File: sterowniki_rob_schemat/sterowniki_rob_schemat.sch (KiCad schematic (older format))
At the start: 6 parts, among them Q1 Q_NPN_BCE, U1 STM32L476VGTx

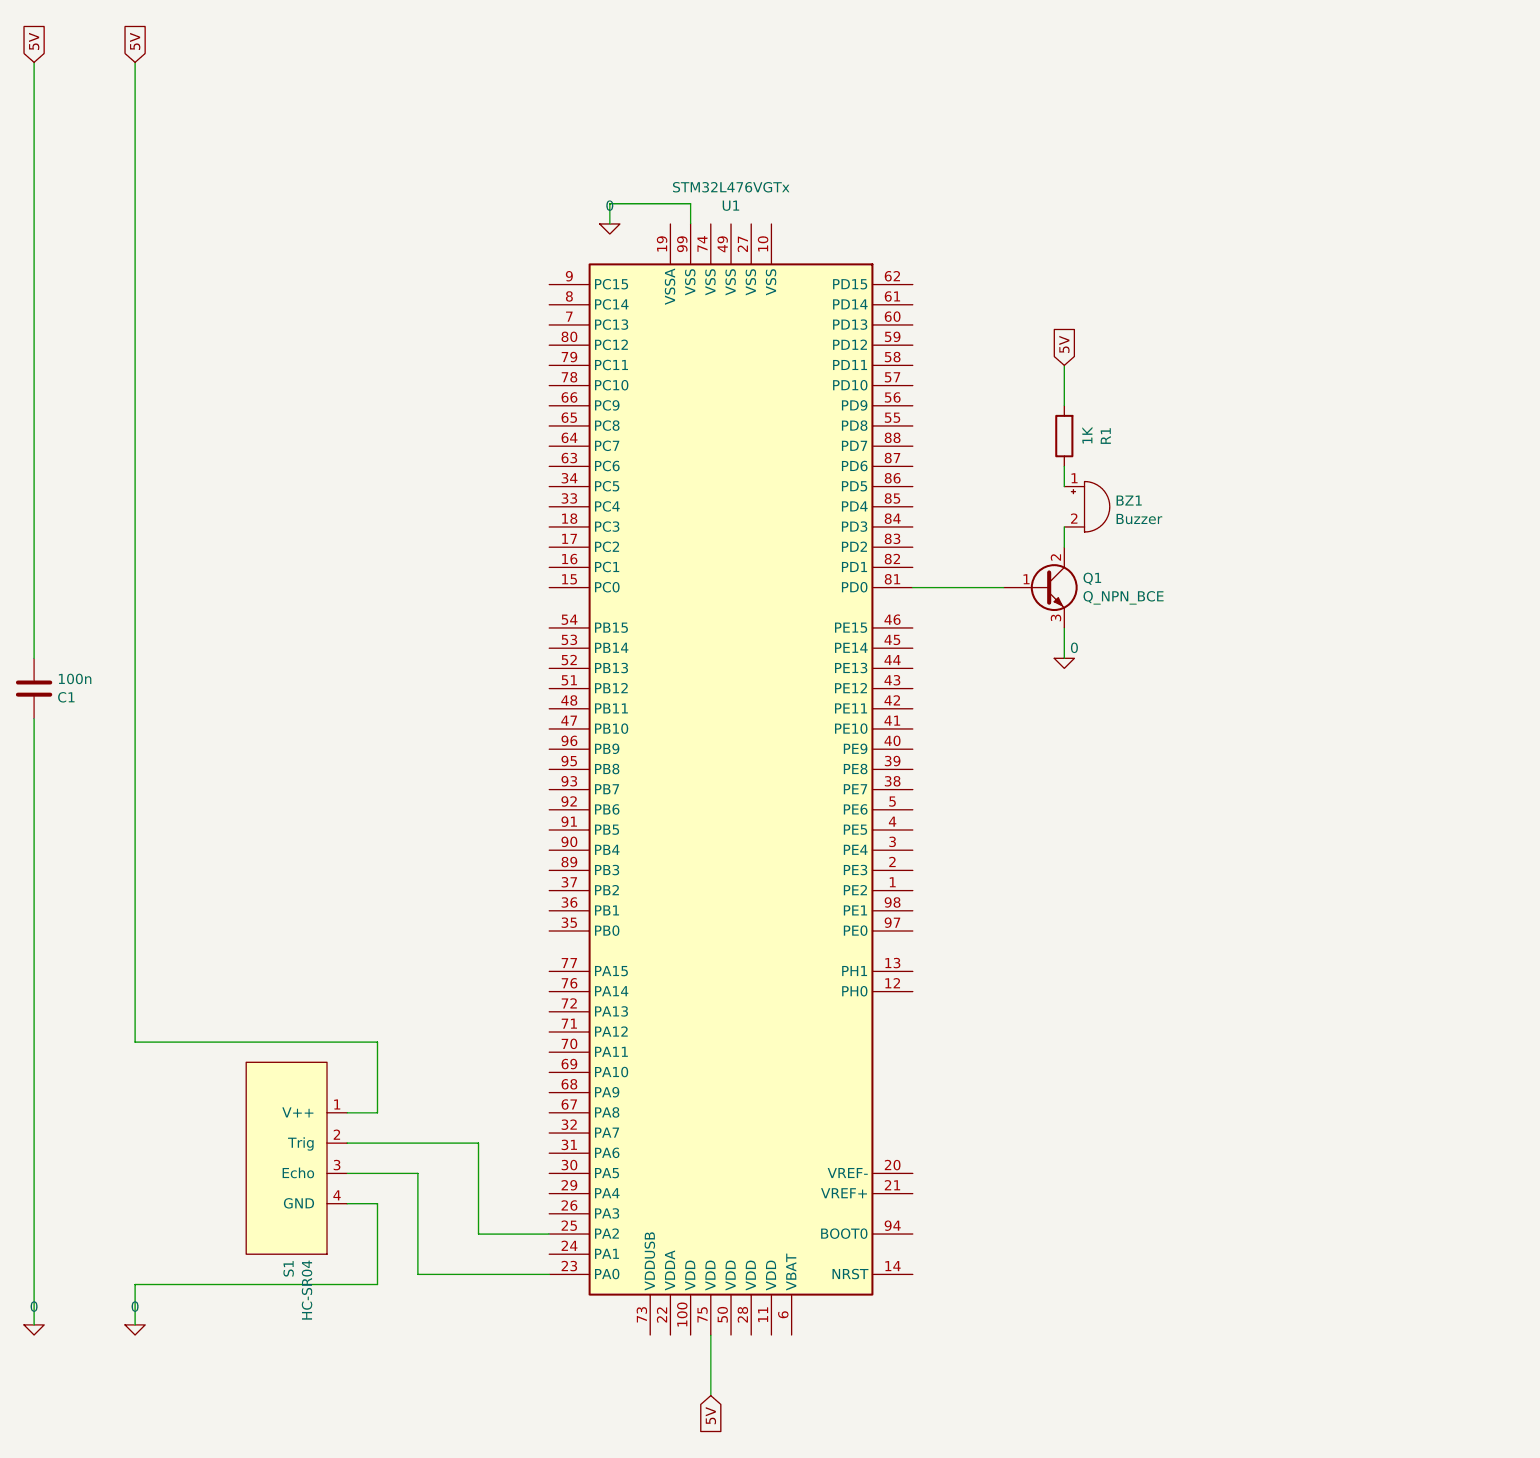
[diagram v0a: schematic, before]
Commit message: końcowy schemat układu
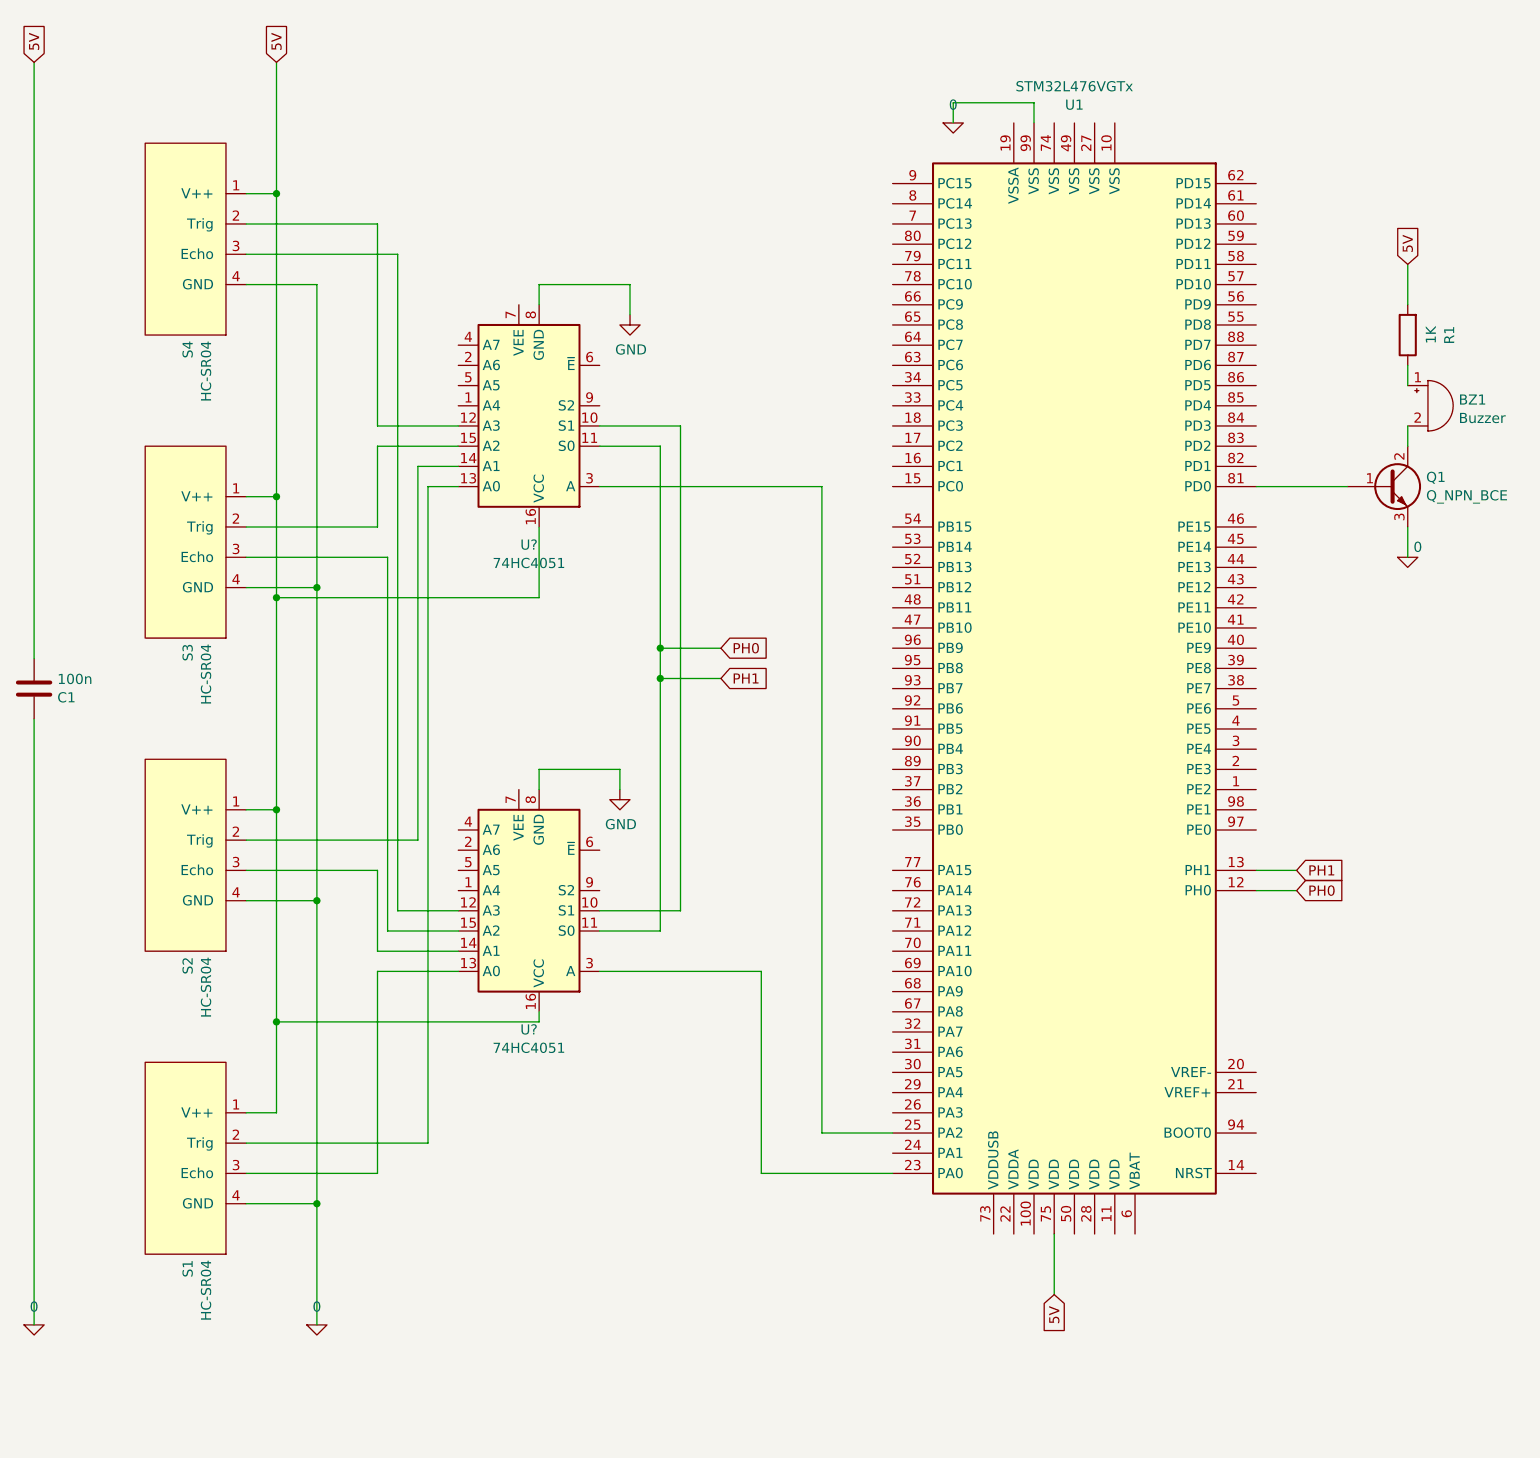
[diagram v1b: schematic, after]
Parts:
- added S2, S3, S4: HC-SR04, symbol bib:HC-SR04
- added U? (x2): 74HC4051, symbol 74xx:74HC4051
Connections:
- net 0: now also S2.4 (GND), S3.4 (GND), S4.4 (GND)
- net 5V: now also S2.1 (V++), S3.1 (V++), S4.1 (V++), U?.16 (VCC), U?.16 (VCC)
- net at S1.2 (Trig): now also U?.13 (A0); no longer U1.25 (PA2)
- net at S1.3 (Echo): now also U?.13 (A0); no longer U1.23 (PA0)
- net PH0: now reaches U1.12 (PH0)
- net PH0: now also U1.13 (PH1), U?.11 (S0), U?.11 (S0)
- new net: U1.23 (PA0), U?.3 (A)
- new net: U1.25 (PA2), U?.3 (A)
- new net: S2.2 (Trig), U?.14 (A1)
- new net: S2.3 (Echo), U?.14 (A1)
- new net: S3.2 (Trig), U?.15 (A2)
- new net: S3.3 (Echo), U?.15 (A2)
- new net: S4.2 (Trig), U?.12 (A3)
- new net: S4.3 (Echo), U?.12 (A3)
- new net: U?.10 (S1), U?.10 (S1)
- new net GND: U?.8 (GND), U?.8 (GND)
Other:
- moved on the sheet: BZ1, Q1, R1, S1, U1
